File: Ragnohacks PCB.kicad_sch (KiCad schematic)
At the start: 35 parts, among them J1 Conn_01x02, J2 Conn_01x18, J3 Conn_01x18, J4 USB_A, SW1 SW_Push, U1 RP2040, U2 W25Q128JVS, U3 LD1117S33TR_SOT223, U4 USBLC6-2P6, Y1 12MHz

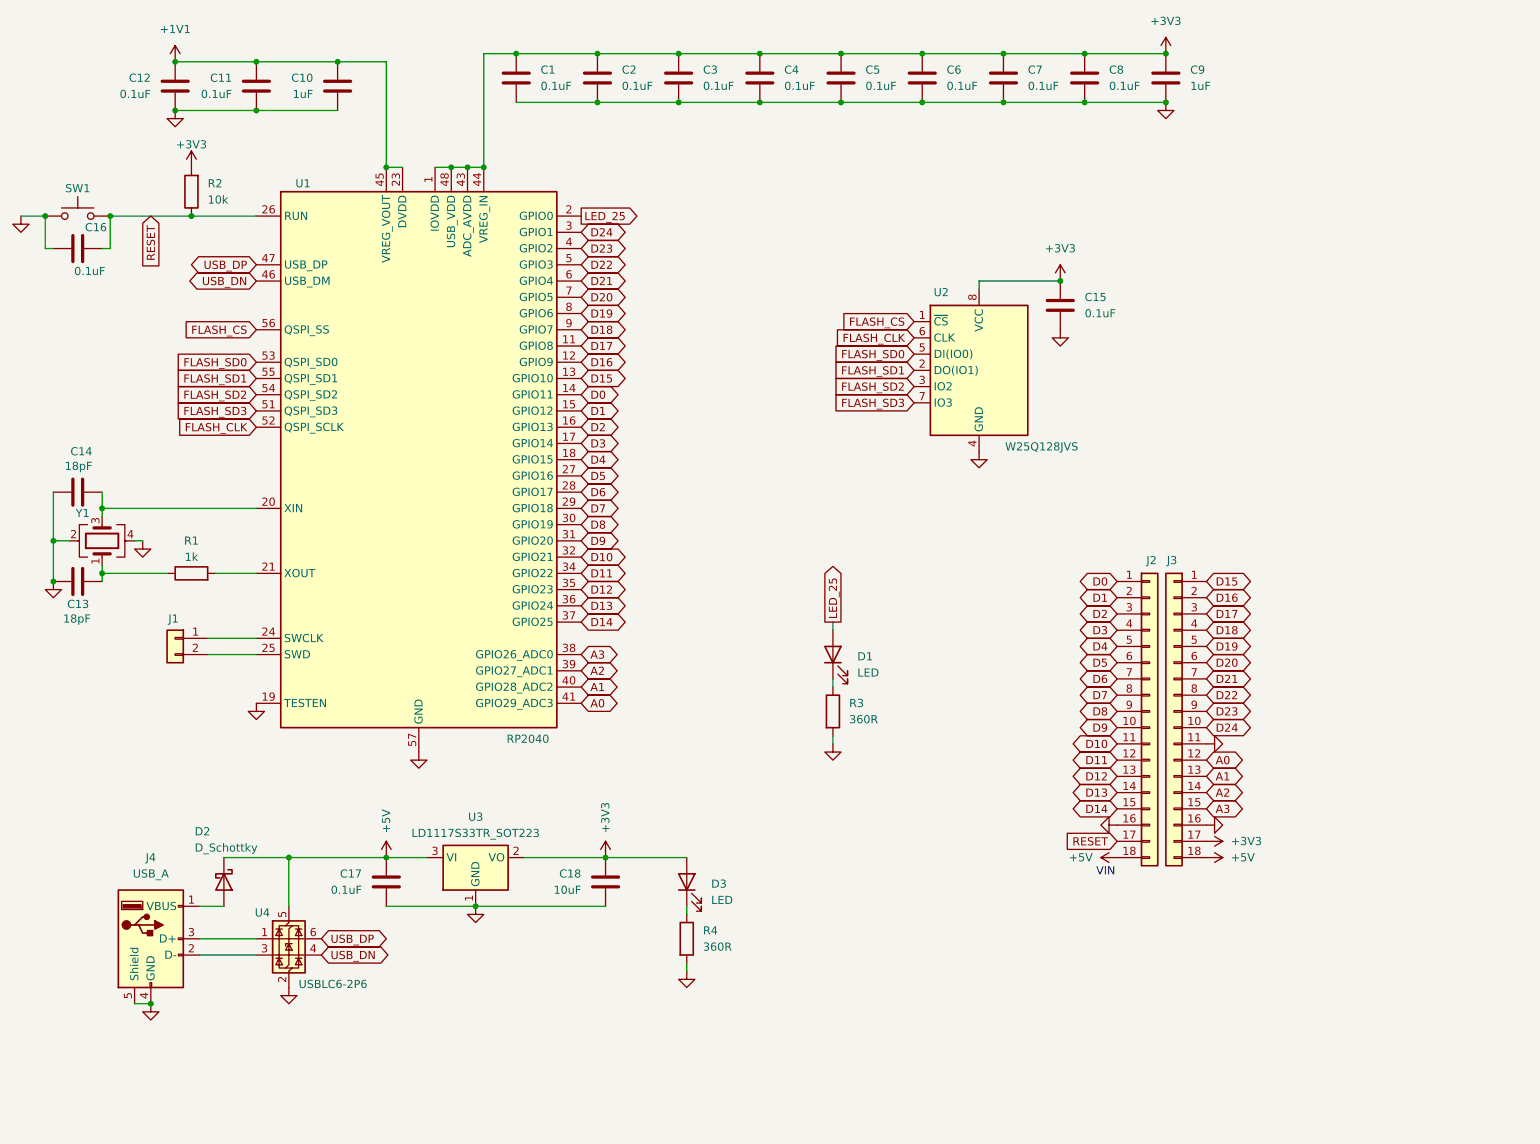
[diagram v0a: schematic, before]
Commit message: Rev 2 of the Ragnohacks PCB
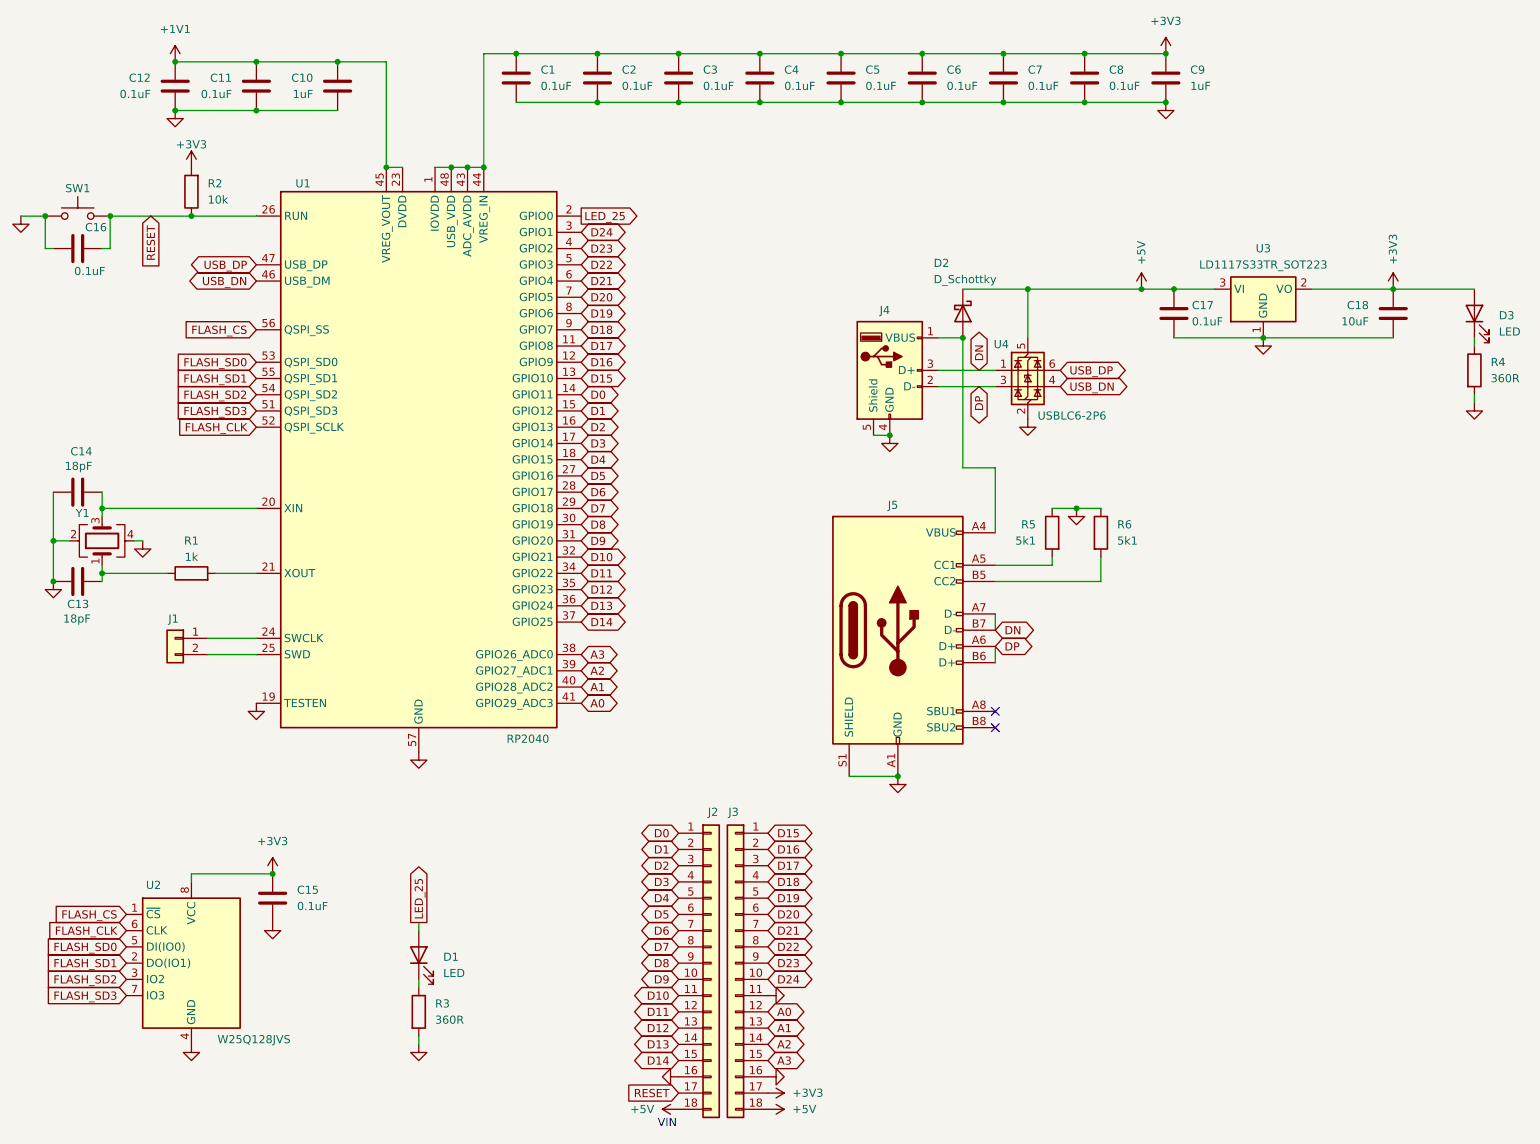
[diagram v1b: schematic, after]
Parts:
- added J5: USB_C_Receptacle_USB2.0_16P, Connector_USB:USB_C_Receptacle_GCT_USB4105-xx-A_16P_TopMnt_Horizontal, symbol Connector:USB_C_Receptacle_USB2.0_16P
- added R5, R6: 5k1, Capacitor_SMD:C_0402_1005Metric, symbol Device:R
- J1: footprint Connector_PinHeader_2.54mm:PinHeader_1x02_P2.54mm_Vertical -> Connector_Wire:SolderWire-2sqmm_1x02_P7.8mm_D2mm_OD3.9mm
- J4: footprint Connector_USB:USB_A_Onboard -> Connector_USB:USB_A_Edge
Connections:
- net GND: now also J5.A1 (GND), J5.A12 (GND), J5.B1 (GND), J5.B12 (GND), J5.S1 (SHIELD), R5.1, R6.1
- net DN: now reaches J4.3 (D+), U4.1 (I/O1)
- net DN: now also J5.A7 (D-), J5.B7 (D-)
- net DP: now reaches J4.2 (D-), U4.3 (I/O2)
- net DP: now also J5.A6 (D+), J5.B6 (D+)
- net at D2.2 (A), J4.1 (VBUS): now also J5.A4 (VBUS), J5.A9 (VBUS), J5.B4 (VBUS), J5.B9 (VBUS)
- new net: J5.A5 (CC1), R5.2
- new net: J5.B5 (CC2), R6.2
- no-connect marks 0 -> 2
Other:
- moved on the sheet: C15, C17, C18, D1, D2, D3, J2, J3, J4, R3, R4, U2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
